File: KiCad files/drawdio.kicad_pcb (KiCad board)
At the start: 2 copper layers, 94 x 22 mm, 26 parts, among them P1 CONN_01X01, P10 CONN_01X02, P2 CONN_01X01, P3 CONN_01X01, P4 CONN_01X02, P5 CONN_01X01, P6 CONN_01X01, P7 CONN_01X01, P9 CONN_02X04, Q1 BC558, Q2 BC547, Q3 BC558, Q4 BC547, U1 LM555N

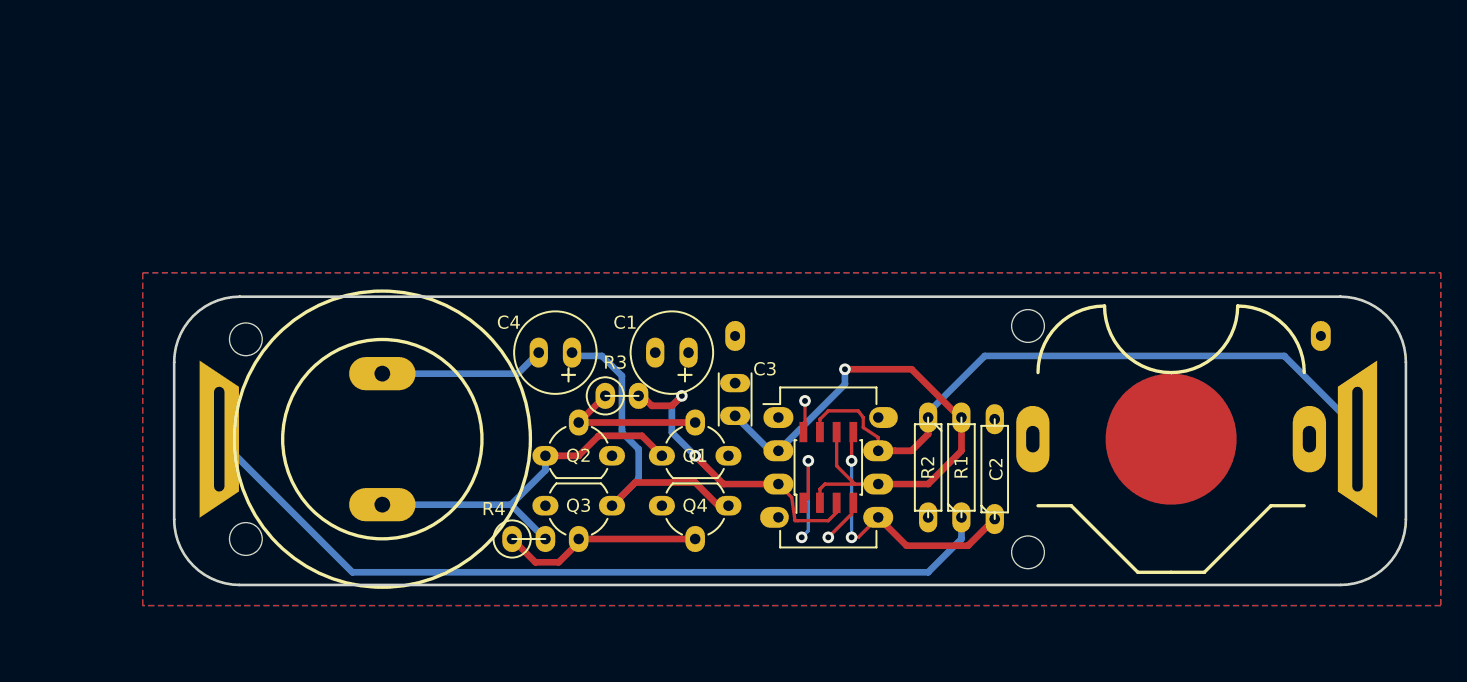
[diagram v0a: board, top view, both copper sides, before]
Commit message: Checkpoint, a dormir!
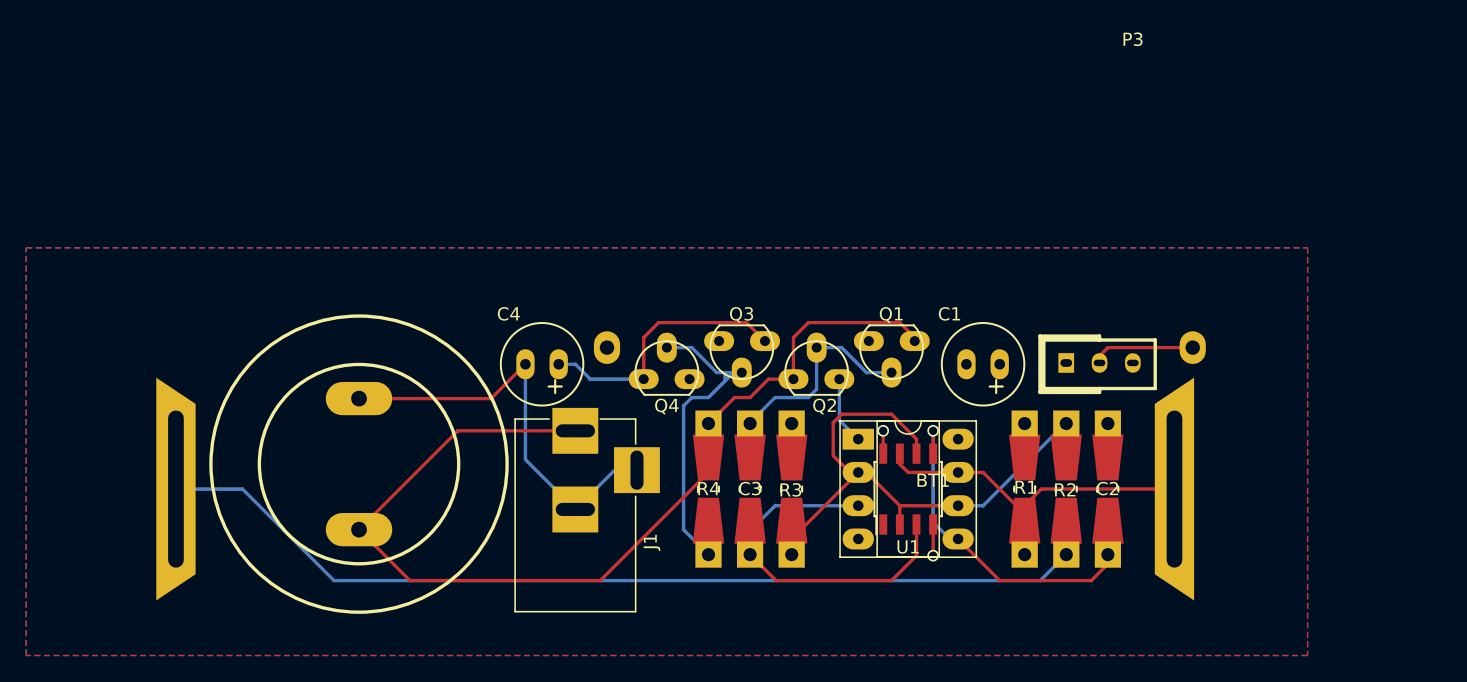
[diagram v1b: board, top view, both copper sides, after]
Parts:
- removed G***: LOGO, uc3music_logos:logo_guitar_22.5x7.7mm_mirror
- removed G***: LOGO, uc3music_logos:logo_pick_15x15mm
- removed G***: LOGO, uc3music_logos:logo_text_20x3.5mm
- removed P10: CONN_01X02, drawdio:AAA_cell_holder
- removed P5, P6, P7: CONN_01X01, Mounting_Holes:MountingHole_2-5mm
- added J1: Jack, Connect:BARREL_JACK, F.Cu at (87.4, 85.7)
- BT1: footprint drawdio:CR2025_Keystone_3002_button_cell_holder_SMT -> AAA_cell_holder
- C1, C4: value CP -> 470uF
- C2: value C -> 0.1uF; footprint Discret:R3 -> Resistors_Universal:Resistor_SMD+THTuniversal_0805to1206_RM10_HandSoldering
- C3: value C -> 680pF; footprint Capacitors_ThroughHole:C_Rect_L4_W2.5_P2.5 -> Resistors_Universal:Resistor_SMD+THTuniversal_0805to1206_RM10_HandSoldering
- P1: value CONN_01X01 -> CON1
- P2: value CONN_01X01 -> CON2
- P3: value CONN_01X01 -> PWR_SW; footprint Mounting_Holes:MountingHole_2-5mm -> drawdio:PWR_SW_Drawdio_SS-12D00(1P2T)
- P4: value CONN_01X02 -> SPK
- Q1, Q2, Q3, Q4: footprint Housings_TO-92:TO-92_Molded_Wide_Oval -> drawdio:TO-92_JorFru_compact
- R1: value R -> 330K; footprint Discret:R3 -> Resistors_Universal:Resistor_SMD+THTuniversal_0805to1206_RM10_HandSoldering
- R2: value R -> 10K; footprint Discret:R3 -> Resistors_Universal:Resistor_SMD+THTuniversal_0805to1206_RM10_HandSoldering
- R3, R4: value R -> 1K; footprint Discret:R1 -> Resistors_Universal:Resistor_SMD+THTuniversal_0805to1206_RM10_HandSoldering
- U1: value LM555N -> NE555; footprint Housings_DIP:DIP-8_W7.62mm_LongPads -> Housings_DIP:DIP-8_W7.62mm_Socket_LongPads
- moved C1 23.8 mm to (119.8, 80.6)
- moved BT1 21.8 mm to (112.1, 79.4)
- moved Q1 20.5 mm to (112.8, 79.4), turned to 180 degrees
- moved Q2 20.4 mm to (104.5, 81.3)
- moved Q3 16.4 mm to (101.3, 79.4)
- moved P3 15.4 mm to (127.4, 80.6), turned to 0 degrees
- moved P2 14.5 mm to (133.1, 90.2)
- moved R4 14.2 mm to (97.5, 90.2), turned to 90 degrees
- moved R3 12.1 mm to (100.7, 90.2), turned to 270 degrees
- moved Q4 11.8 mm to (93.1, 81.3), turned to 0 degrees
- moved C2 8.77 mm to (128.0, 90.2)
- moved R1 8.17 mm to (124.8, 90.2)
- moved R2 7.55 mm to (121.7, 90.2)
- moved C3 7.06 mm to (103.9, 90.2)
- moved P9 6.32 mm to (112.8, 90.2)
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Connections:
- BT1 pad 1: VCC -> Net-(BT1-Pad1)
- P3 pad 1: Net-(P3-Pad1) -> VCC
- R2 pad 1: /pin7 -> VCC
- R2 pad 2: VCC -> /pin7
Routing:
- net Net-(J1-Pad1): track 28.7 -> 77.4 mm
- net /pin7: track 54.6 -> 28.1 mm
- net Net-(C4-Pad2): track 12.6 -> 32.4 mm
- net Net-(Q3-Pad2): track 15.6 -> 27.4 mm
- net Net-(P1-Pad1): track 64.1 -> 74.2 mm
- net Net-(BT1-Pad1): track 0.00 -> 7.91 mm
- net Net-(Q1-Pad2): track 11.8 -> 18.5 mm
- net /pin5: track 21.4 -> 27.7 mm, vias 2 -> 1
- net Net-(C4-Pad1): track 26.2 -> 21.0 mm
- net /pin3: track 25.2 -> 30.1 mm, vias 2 -> 0
- net /pin2: track 43.3 -> 48.0 mm, vias 1 -> 0
- net GND: track 9.42 -> 10.4 mm, vias 2 -> 0
- net VCC: track 5.86 -> 6.71 mm
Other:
- board outline removed
- net class gf: trace_width 0.508 -> 0.254
- board text removed: "Drawdio"
- board text removed: "V1.0"
